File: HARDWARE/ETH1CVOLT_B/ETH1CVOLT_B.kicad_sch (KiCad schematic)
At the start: 0 parts

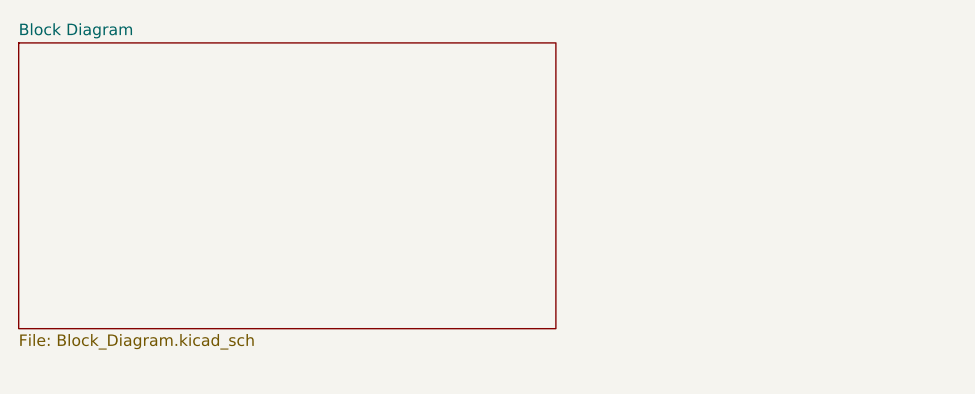
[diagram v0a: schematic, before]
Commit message: Development
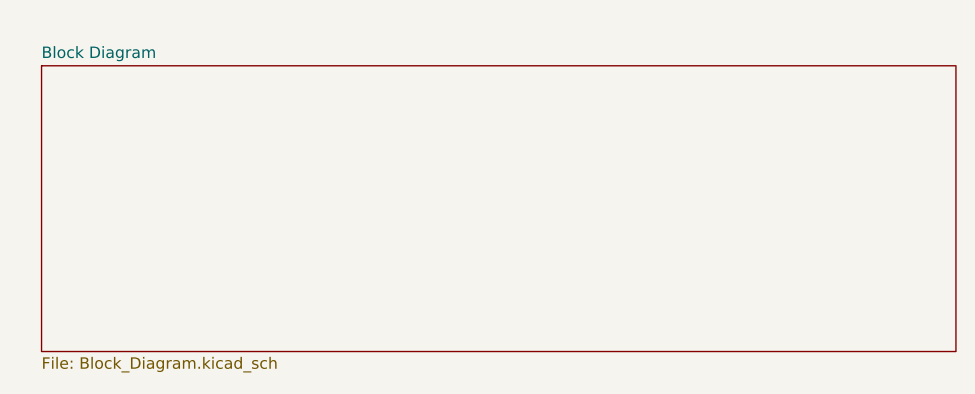
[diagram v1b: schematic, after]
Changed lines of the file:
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@@
 	(paper "A3")
 	(sheet
-		(at 297.18 212.09)
-		(size 59.69 31.75)
+		(at 299.72 214.63)
+		(size 101.6 31.75)
 		(exclude_from_sim no)
 		(in_bom yes)
@@
 		)
 		(property "Sheetname" "Block Diagram"
-			(at 297.18 211.3784 0)
+			(at 299.72 213.9184 0)
 			(effects
 				(font
@@
 		)
 		(property "Sheetfile" "Block_Diagram.kicad_sch"
-			(at 297.18 244.4246 0)
+			(at 299.72 246.9646 0)
 			(effects
 				(font
